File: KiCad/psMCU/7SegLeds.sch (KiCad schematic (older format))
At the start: 14 parts

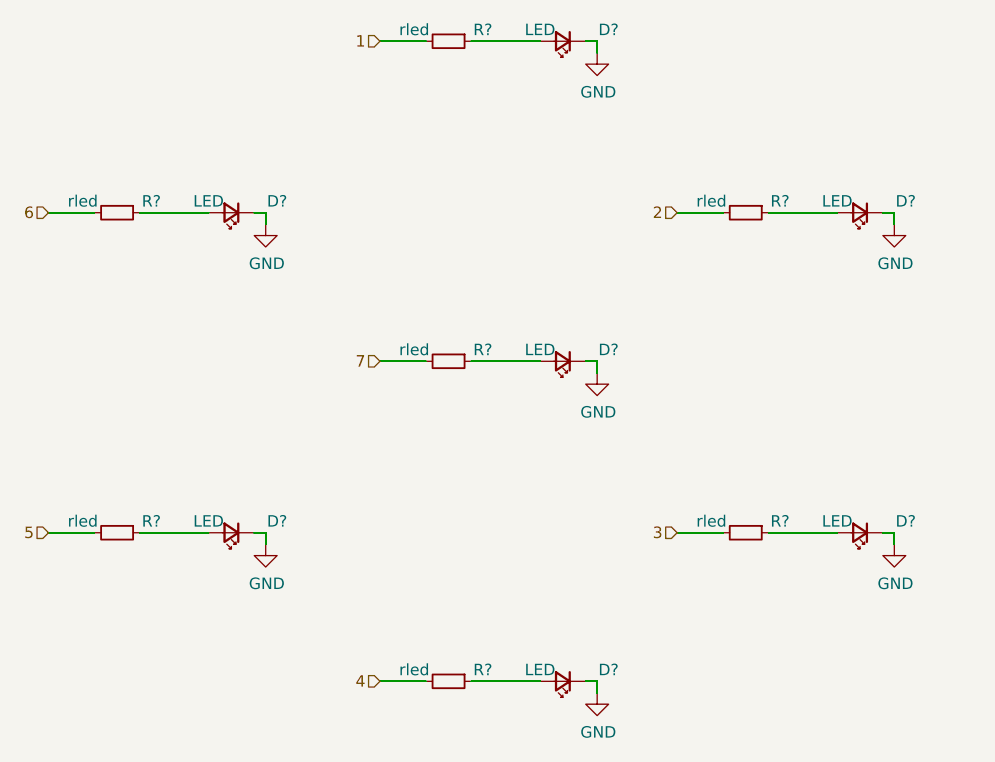
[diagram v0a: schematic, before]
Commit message: First Schematic Draft done.
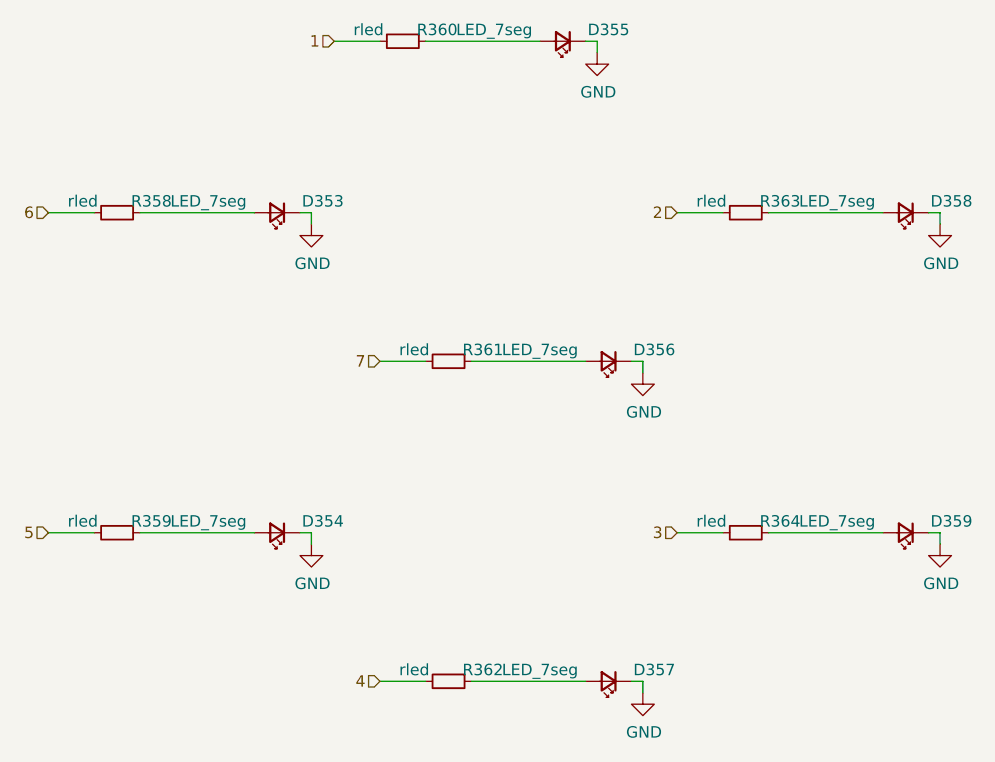
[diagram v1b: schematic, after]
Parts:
- removed D? (x6): LED, Diode_SMD:D_0603_1608Metric, symbol Device:LED_Small
- added D34, D35, D37, D38, D39, D40: LED_7seg, NoRef_Footprints:D_0402_1005Metric_NoRef, symbol Device:LED_Small
- D36: renamed from D?; value LED -> LED_7seg; footprint Diode_SMD:D_0603_1608Metric -> NoRef_Footprints:D_0402_1005Metric_NoRef
- R36, R37, R38, R39, R40, R41, R42: renamed from R?; footprint Resistor_SMD:R_0603_1608Metric -> NoRef_Footprints:R_0603_1608Metric
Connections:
- net GND: now also D34.1 (K), D35.1 (K), D37.1 (K), D38.1 (K), D39.1 (K), D40.1 (K)
- net at R37.1: now also D35.2 (A)
- net at R41.1: now also D39.2 (A)
- net at R40.1: now also D38.2 (A)
- net at R36.1: now also D34.2 (A)
- net at R39.1: now also D37.2 (A)
- net at R42.1: now also D40.2 (A)
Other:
- moved on the sheet: R360
